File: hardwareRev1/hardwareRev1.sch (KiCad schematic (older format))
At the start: 58 parts, among them J1 MicroSD, J2 SMA, K1 PWMOut, K2 ADC1, P1 UART, P10 ID, P2 I2C, P3 ADC2, P4 CONN_7, P5 CONN_5X2, P6 CONN_11X2, P7 GPSDM, P8 GPSDP, P9 USBPW, Q1 MOS_P_NUM, U1 MKL26Z128VLH4, U2 24C16, U3 MICRO-B_USB, X1 CRYSTAL_ABM3C

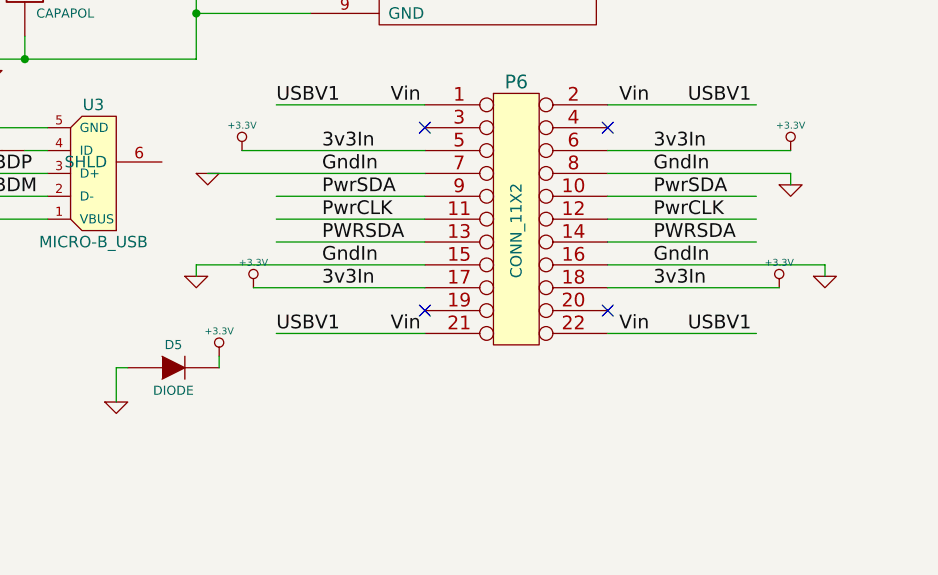
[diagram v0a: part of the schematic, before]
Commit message: went further.
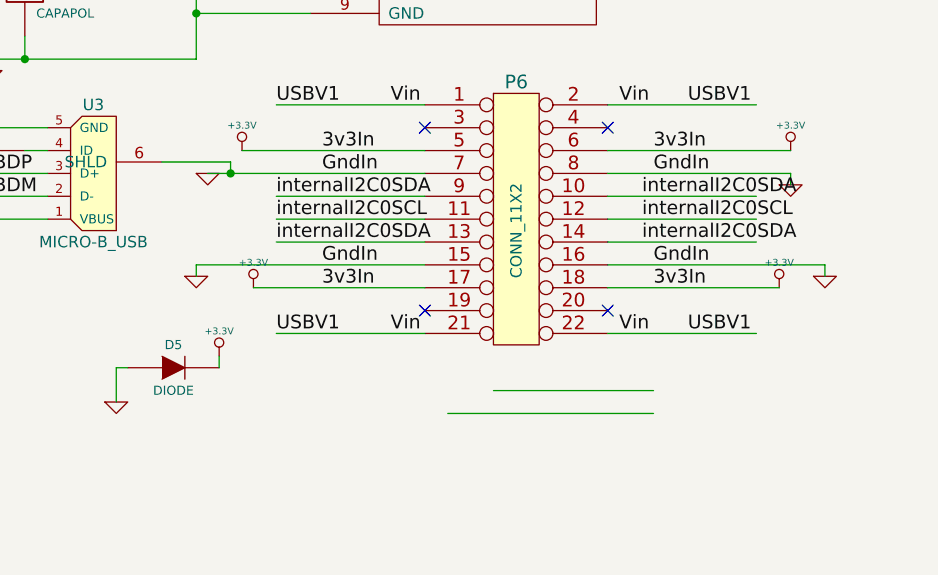
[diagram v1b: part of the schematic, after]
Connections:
- net labels removed: PWRSDA, PwrCLK, PwrSDA
- wire segments 318 -> 322

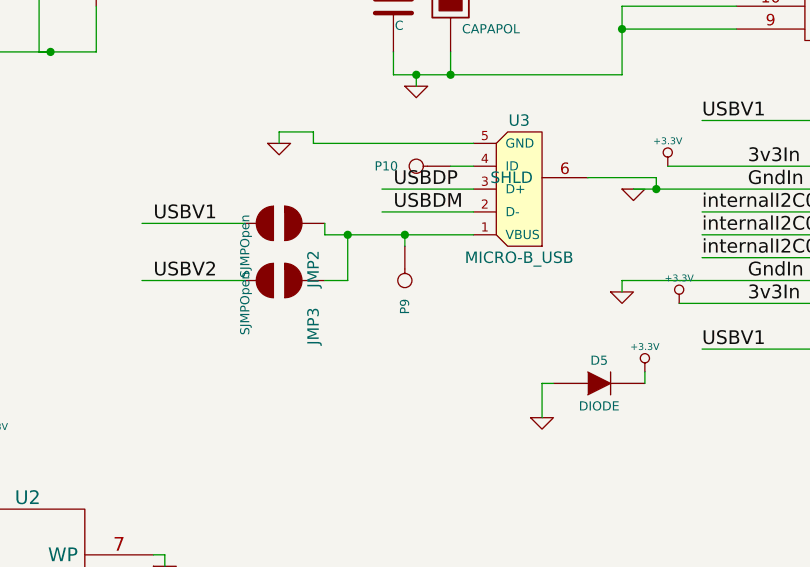
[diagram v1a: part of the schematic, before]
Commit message: better routed it.
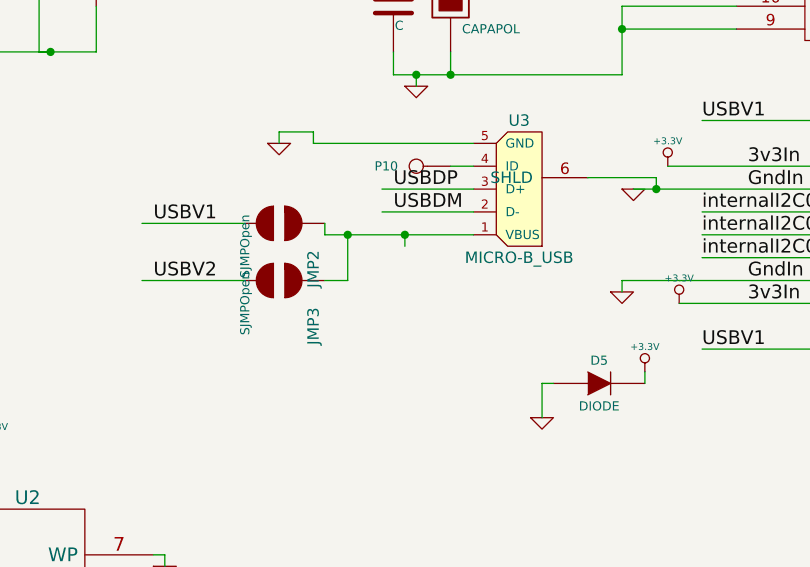
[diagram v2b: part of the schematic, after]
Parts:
- removed P9: USBPW, Measurement_Points:Measurement_Point_Round-SMD-Pad_Small, symbol CONN_1
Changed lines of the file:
@@
 EESchema Schematic File Version 2
+LIBS:hardwareRev1-rescue
 LIBS:power
 LIBS:device
@@
 LIBS:contrib
 LIBS:valves
+LIBS:MKL26Z128VLH4
+LIBS:USB
+LIBS:sma
+LIBS:DataStorage
+LIBS:dra818Real
+LIBS:SparkFun
+LIBS:neo7
+LIBS:gpsant
+LIBS:open-project
+LIBS:smtJmpOpen
 LIBS:conn_11x2
-LIBS:tps63020
-LIBS:ncp508
-LIBS:smtJmpOpen
-LIBS:SparkFun
-LIBS:attiny24a-m
-LIBS:power-cache
+LIBS:MOS_P_NUM
+LIBS:hardwareRev1-cache
 EELAYER 25 0
 EELAYER END
@@
 SW0
 $Comp
-L CONN_1 P9
-U 1 1 554D49E1
-P 7250 5700
-F 0 "P9" H 7330 5700 40  0000 L CNN
-F 1 "USBPW" H 7250 5755 30  0001 C CNN
-F 2 "Measurement_Points:Measurement_Point_Round-SMD-Pad_Small" H 7250 5700 60  0001 C CNN
-F 3 "" H 7250 5700 60  0000 C CNN
-	1    7250 5700
-	0    1    1    0
-$EndComp
-$Comp
 L CONN_1 P10
